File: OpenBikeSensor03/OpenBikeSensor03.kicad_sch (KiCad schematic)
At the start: 24 parts, among them J1 Battery, J2 Ein/Aus-Schalter, J3 Sensor 1, J4 Sensor 2, J5 SD_Card, J6 GPS, J7 Display Cable, J8 Addons, M1 LIPoChargerwithProtection, U1 ESP32 WROOM 30-Pin, U2 DCDC_fix

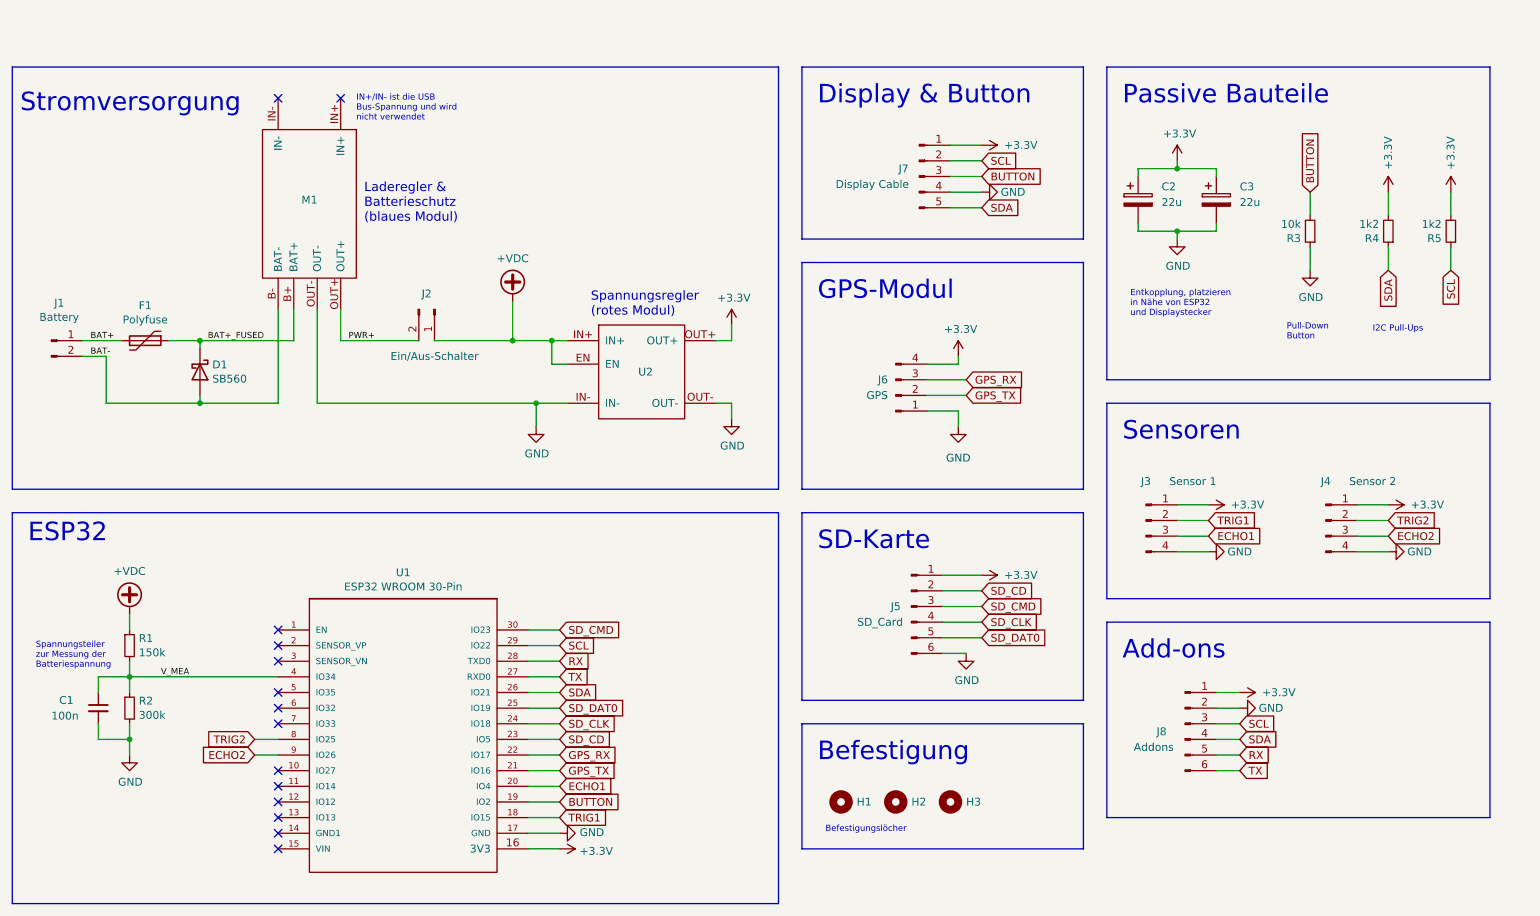
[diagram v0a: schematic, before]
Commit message: clean up libraries
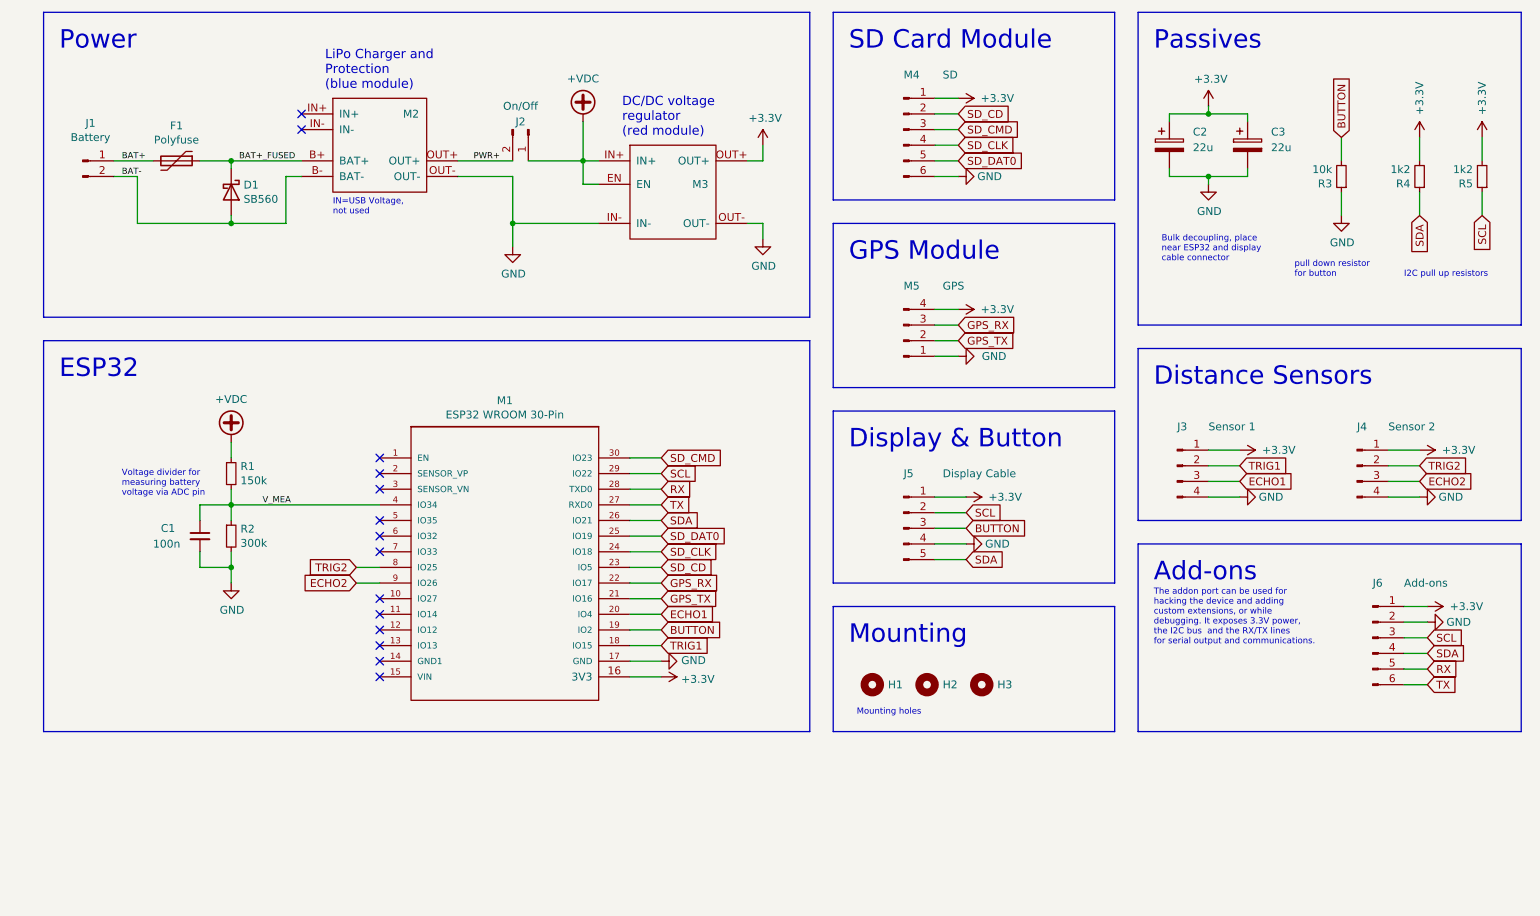
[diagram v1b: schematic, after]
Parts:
- J2: value Ein/Aus-Schalter -> On/Off
- J3, J4: footprint Connector_PinHeader_2.54mm:PinHeader_1x04_P2.54mm_Vertical -> Custom_Modules:Connector_1x04
- J5: renamed from J7; footprint Connector_JST:JST_XH_B5B-XH-AM_1x05_P2.50mm_Vertical -> Custom_Modules:Connector_1x05_Display
- J6: renamed from J8; value Addons -> Add-ons; footprint Connector_PinHeader_2.54mm:PinHeader_1x06_P2.54mm_Vertical -> Custom_Modules:Connector_1x06
- M1: renamed from U1; footprint ESP32-DEVKITC-32D:MODULE_ESP32-DEVKITC-32C_SMD_BOTH -> Custom_Modules:ESP32_WROOM_30_SMD; symbol ESP32-DEVKITC-32D:ESP32-DEVKIT-32C -> Custom_Module:ESP32-WROOM-30
- M2: renamed from M1; symbol Custom_Module:LIPoChargerwithProtection -> Custom_Module:LIPoChargerWithProtection
- M3: renamed from U2; symbol DCDC_Converter:DCDC_fix -> Custom_Module:VoltageRegulator
- M4: renamed from J5; value SD_Card -> SD; footprint Connector_PinHeader_2.54mm:PinHeader_1x06_P2.54mm_Vertical -> Custom_Modules:Connector_1x06
- M5: renamed from J6; footprint Connector_PinHeader_2.54mm:PinHeader_1x04_P2.54mm_Vertical -> Custom_Modules:Connector_1x04
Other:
- note added: "Bulk decoupling, place near ESP32 and display cable connector"
- note added: "DC/DC voltage regulator (red module)"
- note added: "Distance Sensors"
- note added: "GPS Module"
- note added: "I2C pull up resistors"
- note added: "IN=USB Voltage, not used"
- note added: "LiPo Charger and Protection (blue module)"
- note added: "Mounting"
- note added: "Mounting holes"
- note added: "Passives"
- note added: "Power"
- note added: "SD Card Module"
- note added: "The addon port can be used for hacking the device and adding custom extensions, or while debugging. It exposes 3.3V power, the I2C bus and the RX/TX lines for serial output and communications."
- note added: "Voltage divider for measuring battery voltage via ADC pin"
- note added: "pull down resistor for button"
- note removed: "Befestigung"
- note removed: "Befestigungslöcher"
- note removed: "Entkopplung, platzieren in Nähe von ESP32 und Displaystecker"
- note removed: "GPS-Modul"
- note removed: "I2C Pull-Ups"
- note removed: "IN+/IN- ist die USB Bus-Spannung und wird nicht verwendet"
- note removed: "Laderegler & Batterieschutz (blaues Modul)"
- note removed: "Passive Bauteile"
- note removed: "Pull-Down Button"
- note removed: "SD-Karte"
- note removed: "Sensoren"
- note removed: "Spannungsregler (rotes Modul)"
- note removed: "Spannungsteiler zur Messung der Batteriespannung"
- note removed: "Stromversorgung"
- moved on the sheet: C1, C2, C3, D1, F1, H1, H2, H3, J1, J2, J3, J4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
